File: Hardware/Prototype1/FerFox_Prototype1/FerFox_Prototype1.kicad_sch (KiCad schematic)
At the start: 33 parts, among them J1 Conn_01x08_Pin, J2 Conn_01x06_Pin, U1 STM32F401CCUx, Y1 25MHz, Y2 32768 Hz

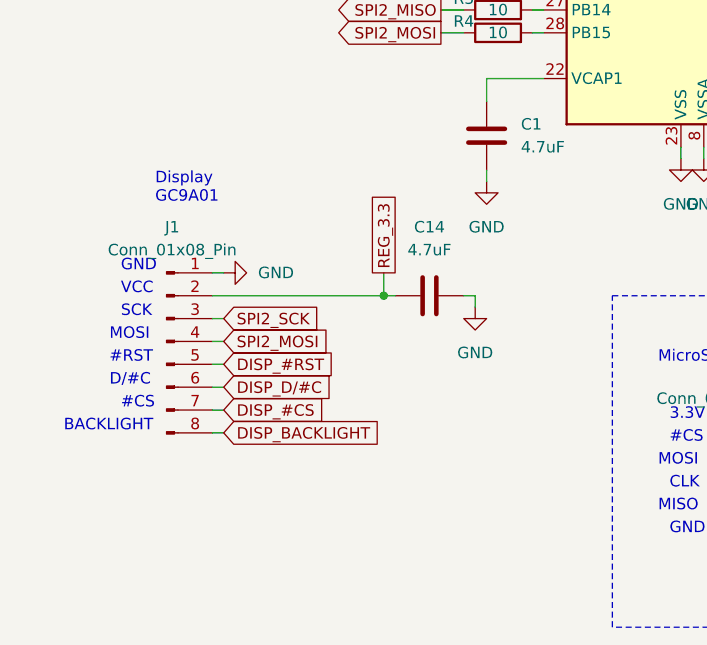
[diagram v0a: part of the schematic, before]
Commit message: Modifications in circuit
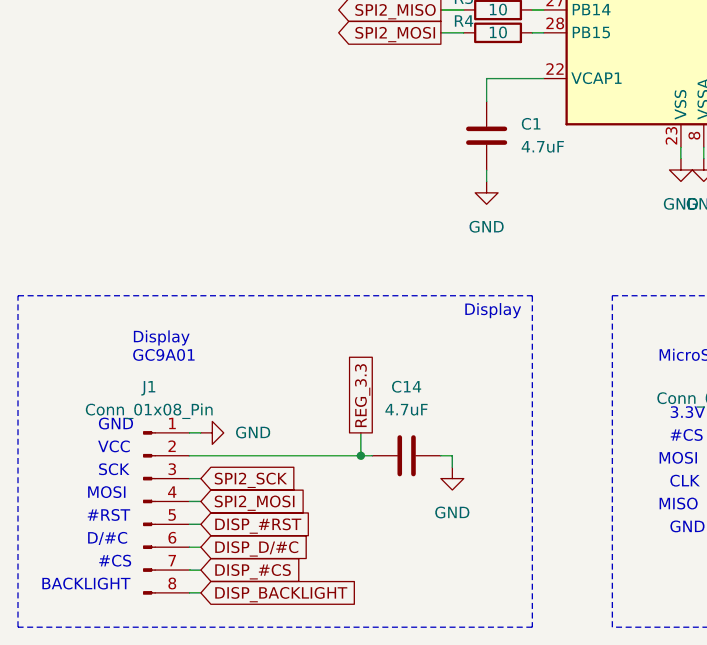
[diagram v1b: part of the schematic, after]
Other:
- note added: "Display"
- moved on the sheet: C14, J1
